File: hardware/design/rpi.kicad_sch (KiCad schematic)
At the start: 3 parts, among them U7 RASPBERRY_PI_ZERO_2_W

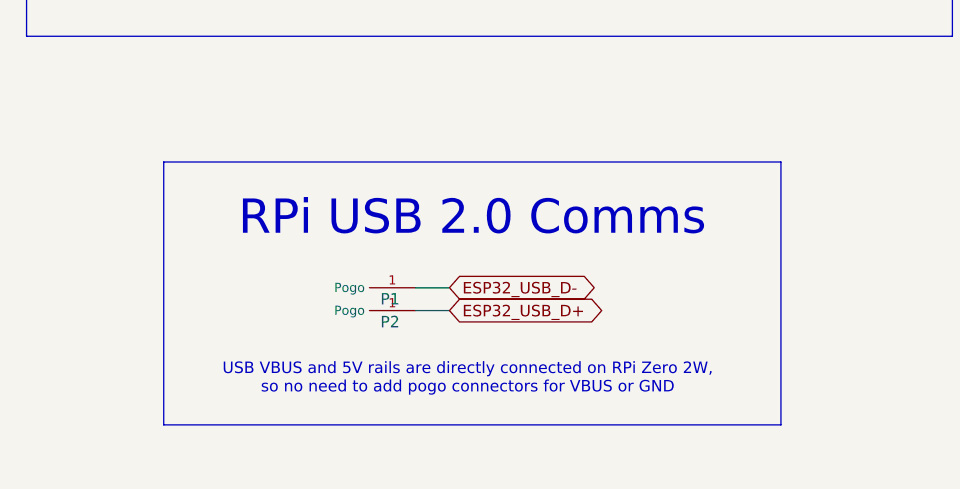
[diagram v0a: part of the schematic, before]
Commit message: Start work on layout
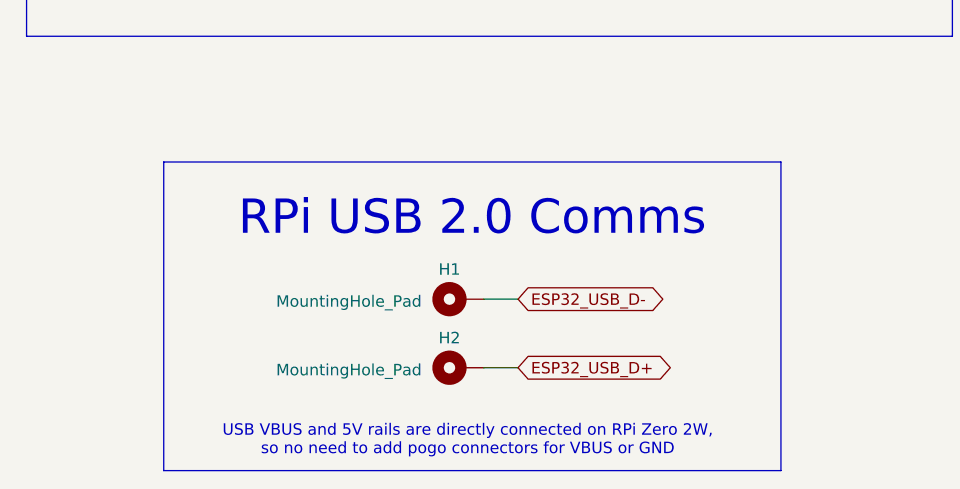
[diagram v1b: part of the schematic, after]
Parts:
- removed P1, P2: ~, symbol CustomLibrary:Pogo_Pin
- added H1, H2: MountingHole_Pad, Connector_PinHeader_2.00mm:PinHeader_1x01_P2.00mm_Vertical, symbol Mechanical:MountingHole_Pad
- U7: footprint RASPBERRY_PI_ZERO_2_W:MODULE_RASPBERRY_PI_ZERO_2_W -> RASPBERRY_PI_ZERO_2_W:Raspberry Pi Zero 2W Header
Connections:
- net ESP32_USB_D+: now also H2.1
- net ESP32_USB_D-: now also H1.1
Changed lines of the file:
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@@
 	(wire
 		(pts
-			(xy 77.47 175.26) (xy 81.28 175.26)
+			(xy 85.09 181.61) (xy 88.9 181.61)
 		)
 		(stroke
@@
 	(wire
 		(pts
-			(xy 77.47 172.72) (xy 81.28 172.72)
+			(xy 85.09 173.99) (xy 88.9 173.99)
 		)
 		(stroke
@@
 	(rectangle
 		(start 49.53 158.75)
-		(end 118.11 187.96)
+		(end 118.11 193.04)
 		(stroke
 			(width 0)
@@
 	(text "USB VBUS and 5V rails are directly connected on RPi Zero 2W,\nso no need to add pogo connectors for VBUS or GND"
 		(exclude_from_sim no)
-		(at 83.312 182.88 0)
+		(at 83.312 189.738 0)
 		(effects
 			(font
@@
 	(global_label "ESP32_USB_D-"
 		(shape bidirectional)
-		(at 81.28 172.72 0)
+		(at 88.9 173.99 0)
 		(fields_autoplaced yes)
 		(effects
@@
 		)
 		(property "Intersheetrefs" "${INTERSHEET_REFS}"
-			(at 100.0116 172.72 0)
+			(at 107.6316 173.99 0)
 			(effects
 				(font
@@
 	(global_label "ESP32_USB_D+"
 		(shape bidirectional)
-		(at 81.28 175.26 0)
+		(at 88.9 181.61 0)
 		(fields_autoplaced yes)
 		(effects
@@
 		)
 		(property "Intersheetrefs" "${INTERSHEET_REFS}"
-			(at 100.0116 175.26 0)
+			(at 107.6316 181.61 0)
 			(effects
 				(font
@@
 	)
 	(symbol
-		(lib_id "CustomLibrary:Pogo_Pin")
-		(at 74.93 173.99 0)
+		(lib_id "Mechanical:MountingHole_Pad")
+		(at 82.55 181.61 90)
 		(unit 1)
-		(exclude_from_sim no)
-		(in_bom yes)
+		(exclude_from_sim yes)
+		(in_bom no)
 		(on_board yes)
 		(dnp no)
-		(property "Reference" "P1"
-			(at 74.676 173.99 0)
-			(effects
-				(font
-					(size 1.27 1.27)
-				)
-			)
-		)
-		(property "Value" "~"
-			(at 72.39 171.45 0)
-			(effects
-				(font
-					(size 1.27 1.27)
-				)
-			)
-		)
-		(property "Footprint" ""
-			(at 74.93 173.99 0)
-			(effects
-				(font
-					(size 1.27 1.27)
-				)
-				(hide yes)
-			)
-		)
-		(property "Datasheet" ""
-			(at 74.93 173.99 0)
-			(effects
-				(font
-					(size 1.27 1.27)
-				)
-				(hide yes)
-			)
-		)
-		(property "Description" ""
-			(at 74.93 173.99 0)
+		(property "Reference" "H2"
+			(at 81.28 178.308 90)
+			(effects
+				(font
+					(size 1.27 1.27)
+				)
+			)
+		)
+		(property "Value" "MountingHole_Pad"
+			(at 70.104 181.864 90)
+			(effects
+				(font
+					(size 1.27 1.27)
+				)
+			)
+		)
+		(property "Footprint" "Connector_PinHeader_2.00mm:PinHeader_1x01_P2.00mm_Vertical"
+			(at 82.55 181.61 0)
+			(effects
+				(font
+					(size 1.27 1.27)
+				)
+				(hide yes)
+			)
+		)
+		(property "Datasheet" "~"
+			(at 82.55 181.61 0)
+			(effects
+				(font
+					(size 1.27 1.27)
+				)
+				(hide yes)
+			)
+		)
+		(property "Description" "Mounting Hole with connection"
+			(at 82.55 181.61 0)
 			(effects
 				(font
@@
 		)
 		(instances
-			(project ""
+			(project "CivicAlert"
 				(path "/3dbd3de8-ad8a-405d-8846-2fd4fec89053/6e34966e-7af6-478b-ab27-6fe42694dcb3"
-					(reference "P1")
-					(unit 1)
-				)
-			)
-		)
-	)
-	(symbol
-		(lib_id "CustomLibrary:Pogo_Pin")
-		(at 74.93 176.53 0)
-		(unit 1)
-		(exclude_from_sim no)
-		(in_bom yes)
-		(on_board yes)
-		(dnp no)
-		(property "Reference" "P2"
-			(at 74.676 176.53 0)
-			(effects
-				(font
-					(size 1.27 1.27)
-				)
-			)
-		)
-		(property "Value" "~"
-			(at 72.39 173.99 0)
-			(effects
-				(font
-					(size 1.27 1.27)
-				)
-			)
-		)
-		(property "Footprint" ""
-			(at 74.93 176.53 0)
-			(effects
-				(font
-					(size 1.27 1.27)
-				)
-				(hide yes)
-			)
-		)
-		(property "Datasheet" ""
-			(at 74.93 176.53 0)
-			(effects
-				(font
-					(size 1.27 1.27)
-				)
-				(hide yes)
-			)
-		)
-		(property "Description" ""
-			(at 74.93 176.53 0)
-			(effects
-				(font
-					(size 1.27 1.27)
-				)
-				(hide yes)
-			)
-		)
-		(pin "1"
-		)
-		(instances
-			(project ""
-				(path "/3dbd3de8-ad8a-405d-8846-2fd4fec89053/6e34966e-7af6-478b-ab27-6fe42694dcb3"
-					(reference "P2")
+					(reference "H2")
 					(unit 1)
 				)
@@
 	)
 	(symbol
+		(lib_id "Mechanical:MountingHole_Pad")
+		(at 82.55 173.99 90)
+		(unit 1)
+		(exclude_from_sim yes)
+		(in_bom no)
+		(on_board yes)
+		(dnp no)
+		(property "Reference" "H1"
+			(at 81.28 170.688 90)
+			(effects
+				(font
+					(size 1.27 1.27)
+				)
+			)
+		)
+		(property "Value" "MountingHole_Pad"
+			(at 70.104 174.244 90)
+			(effects
+				(font
+					(size 1.27 1.27)
+				)
+			)
+		)
+		(property "Footprint" "Connector_PinHeader_2.00mm:PinHeader_1x01_P2.00mm_Vertical"
+			(at 82.55 173.99 0)
+			(effects
+				(font
+					(size 1.27 1.27)
+				)
+				(hide yes)
+			)
+		)
+		(property "Datasheet" "~"
+			(at 82.55 173.99 0)
+			(effects
+				(font
+					(size 1.27 1.27)
+				)
+				(hide yes)
+			)
+		)
+		(property "Description" "Mounting Hole with connection"
+			(at 82.55 173.99 0)
+			(effects
+				(font
+					(size 1.27 1.27)
+				)
+				(hide yes)
+			)
+		)
+		(pin "1"
+		)
+		(instances
+			(project ""
+				(path "/3dbd3de8-ad8a-405d-8846-2fd4fec89053/6e34966e-7af6-478b-ab27-6fe42694dcb3"
+					(reference "H1")
+					(unit 1)
+				)
+			)
+		)
+	)
+	(symbol
 		(lib_id "RASPBERRY_PI_ZERO_2_W:RASPBERRY_PI_ZERO_2_W")
 		(at 74.93 96.52 0)
@@
 			)
 		)
-		(property "Footprint" "RASPBERRY_PI_ZERO_2_W:MODULE_RASPBERRY_PI_ZERO_2_W"
+		(property "Footprint" "RASPBERRY_PI_ZERO_2_W:Raspberry Pi Zero 2W Header"
 			(at 74.93 96.52 0)
 			(effects
